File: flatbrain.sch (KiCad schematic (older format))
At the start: 89 parts, among them J1 OLED, J2 Conn_01x05, SW1 Rotary_Encoder_Switch, SW2 Rotary_Encoder_Switch, U1 Elite-C

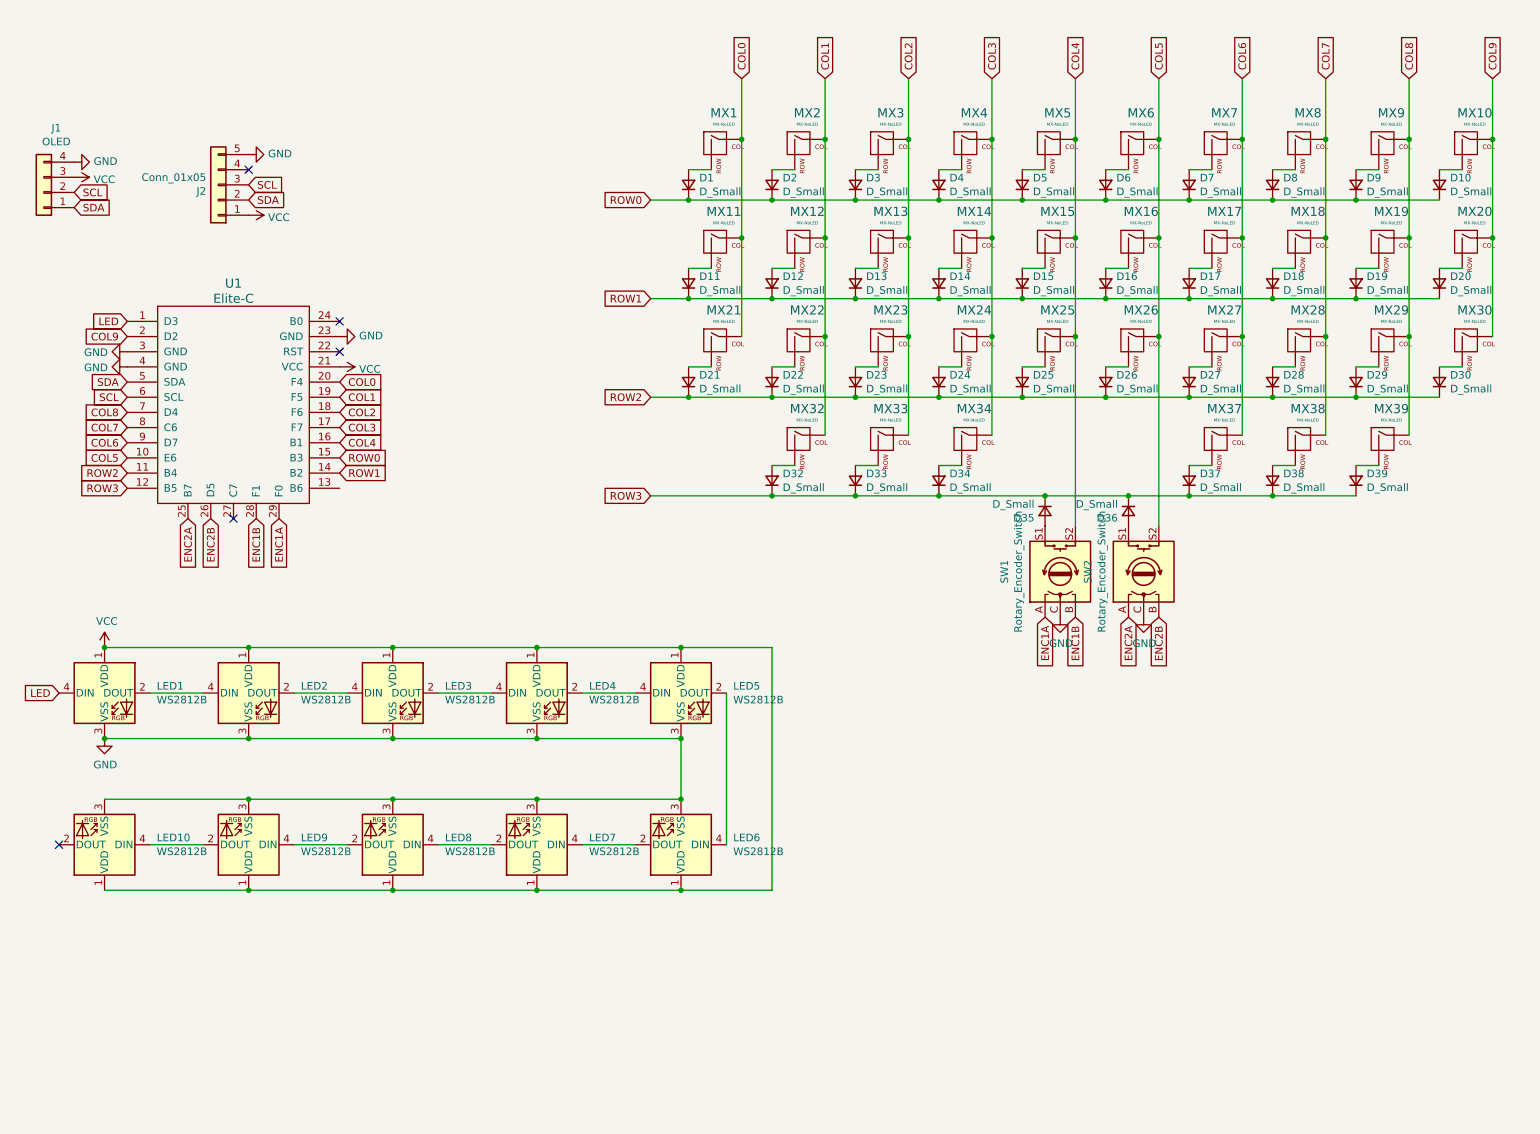
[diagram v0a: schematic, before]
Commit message: half pcba
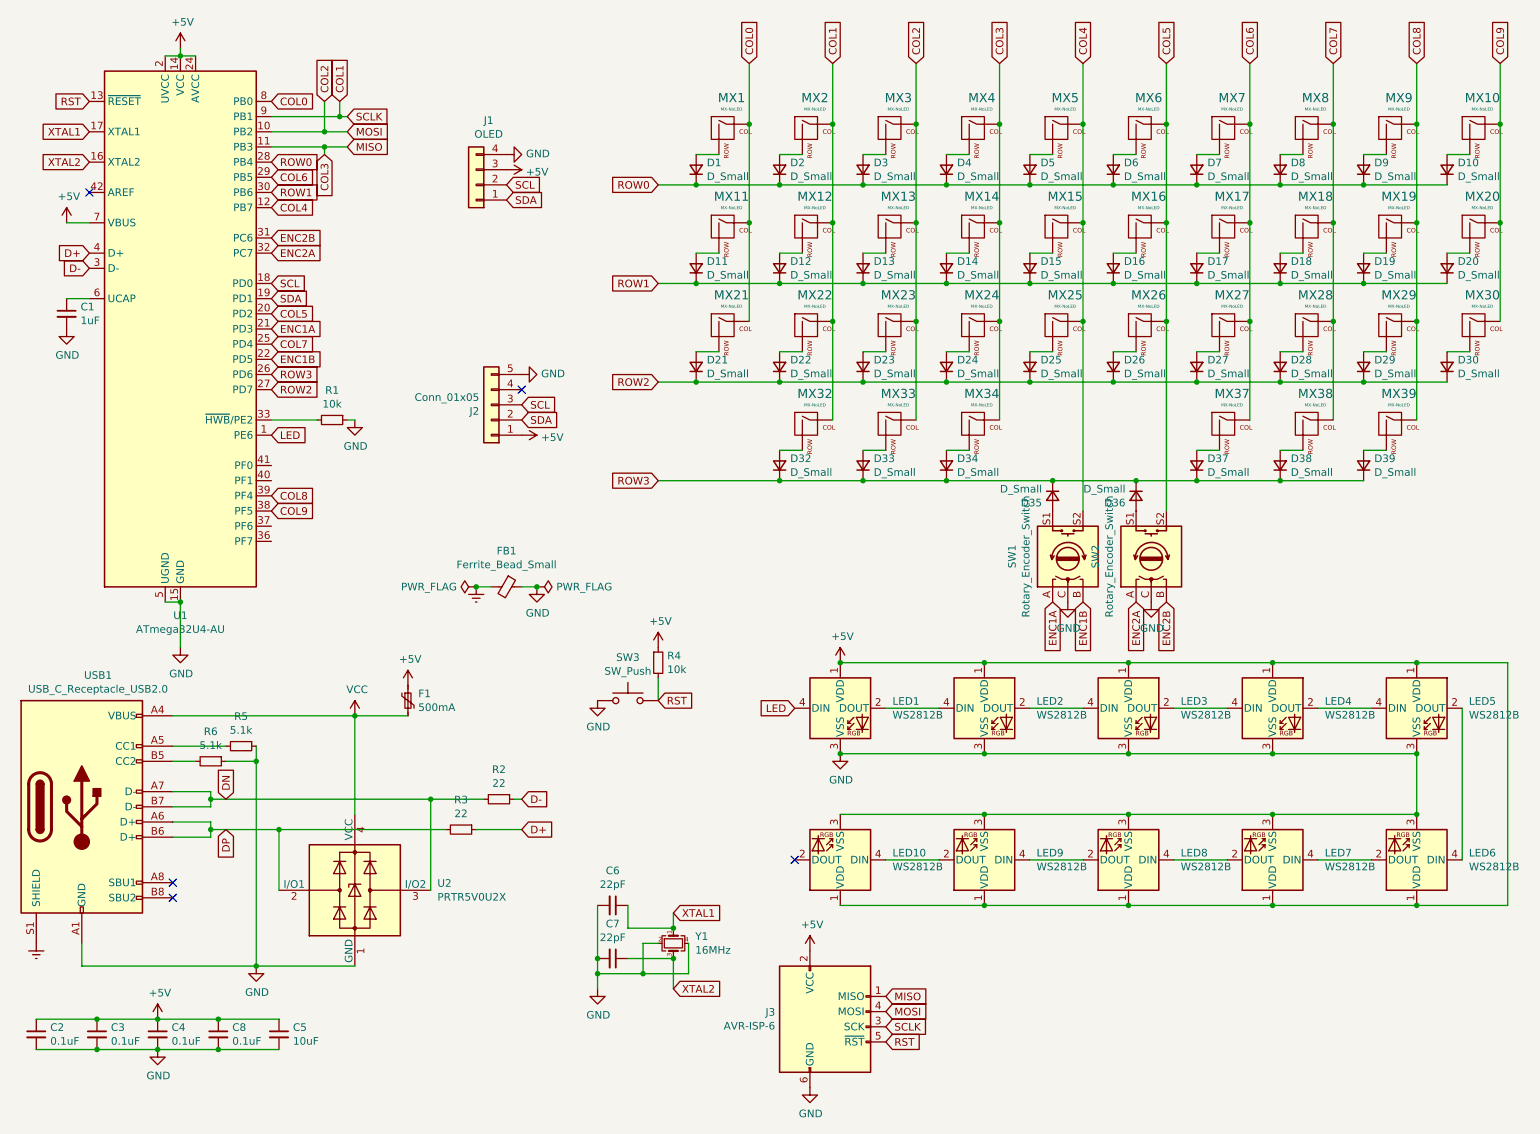
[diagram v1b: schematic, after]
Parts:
- removed U1: Elite-C, Keebio-Parts:Elite-C, symbol flatbrain:Elite-C
- added C1: 1uF, Capacitor_SMD:C_0805_2012Metric, symbol Device:C_Small
- added C2, C3, C4, C8: 0.1uF, Capacitor_SMD:C_0805_2012Metric, symbol Device:C_Small
- added C5: 10uF, Capacitor_SMD:C_0805_2012Metric, symbol Device:C_Small
- added C6, C7: 22pF, Capacitor_SMD:C_0805_2012Metric, symbol Device:C_Small
- added F1: 500mA, Fuse:Fuse_1206_3216Metric, symbol Device:Polyfuse_Small
- added FB1: Ferrite_Bead_Small, Inductor_SMD:L_0805_2012Metric_Pad1.15x1.40mm_HandSolder, symbol Device:Ferrite_Bead_Small
- added J3: AVR-ISP-6, random-keyboard-parts:Reset_Pretty-Mask, symbol Connector:AVR-ISP-6
- added R1, R4: 10k, Resistor_SMD:R_0805_2012Metric, symbol Device:R_Small
- added R2, R3: 22, Resistor_SMD:R_0805_2012Metric, symbol Device:R_Small
- added R5, R6: 5.1k, Resistor_SMD:R_0805_2012Metric, symbol Device:R_Small
- added SW3: SW_Push, random-keyboard-parts:SKQG-1155865, symbol Switch:SW_Push
- added U1: ATmega32U4-AU, Package_QFP:TQFP-44_10x10mm_P0.8mm, symbol MCU_Microchip_ATmega:ATmega32U4-AU
- added U2: PRTR5V0U2X, random-keyboard-parts:SOT143B, symbol Power_Protection:PRTR5V0U2X
- added USB1: USB_C_Receptacle_USB2.0, Connector_USB:USB_C_Receptacle_HRO_TYPE-C-31-M-12, symbol Connector:USB_C_Receptacle_USB2.0
- added Y1: 16MHz, Crystal:Crystal_SMD_3225-4Pin_3.2x2.5mm, symbol Device:Crystal_GND24_Small
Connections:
- net COL0: now also U1.8 (PB0)
- net COL1: now also J3.3 (SCK), U1.9 (PB1)
- net COL2: now also J3.4 (MOSI), U1.10 (PB2)
- net COL3: now also J3.1 (MISO), U1.11 (PB3)
- net COL4: now also U1.12 (PB7)
- net COL5: now also U1.20 (PD2)
- net COL6: now also U1.29 (PB5)
- net COL7: now also U1.25 (PD4)
- net COL8: now also U1.39 (PF4)
- net COL9: now also U1.38 (PF5)
- net ENC1A: now also U1.21 (PD3)
- net ENC1B: now also U1.22 (PD5)
- net ENC2A: now also U1.32 (PC7)
- net ENC2B: now also U1.31 (PC6)
- net GND: now also C1.2, C2.2, C3.2, C4.2, C5.2, C6.2, C7.2, C8.2, FB1.1, J3.6 (GND), R1.1, R5.1, R6.1, SW3.1, U1.15 (GND), U1.23 (GND), U1.35 (GND), U1.43 (GND), U1.5 (UGND), U2.1 (GND), USB1.A1 (GND), USB1.A12 (GND), USB1.B1 (GND), USB1.B12 (GND), Y1.2, Y1.4
- net LED: now also U1.1 (PE6)
- net ROW0: now also U1.28 (PB4)
- net ROW1: now also U1.30 (PB6)
- net ROW2: now also U1.27 (PD7)
- net ROW3: now also U1.26 (PD6)
- net SCL: now also U1.18 (PD0)
- net SDA: now also U1.19 (PD1)
- net VCC: now also F1.2, U2.4 (VCC), USB1.A4 (VBUS), USB1.A9 (VBUS), USB1.B4 (VBUS), USB1.B9 (VBUS); no longer J1.3 (Pin_3), J2.1 (Pin_1), LED1.1 (VDD), LED10.1 (VDD), LED2.1 (VDD), LED3.1 (VDD), LED4.1 (VDD), LED5.1 (VDD), LED6.1 (VDD), LED7.1 (VDD), LED8.1 (VDD), LED9.1 (VDD)
- new net: R1.2, U1.33 (~HWB~/PE2)
- new net: C1.1, U1.6 (UCAP)
- new net: R5.2, USB1.A5 (CC1)
- new net: R6.2, USB1.B5 (CC2)
- new net +5V: C2.1, C3.1, C4.1, C5.1, C8.1, F1.1, J1.3 (Pin_3), J2.1 (Pin_1), J3.2 (VCC), LED1.1 (VDD), LED10.1 (VDD), LED2.1 (VDD), LED3.1 (VDD), LED4.1 (VDD), LED5.1 (VDD), LED6.1 (VDD), LED7.1 (VDD), LED8.1 (VDD), LED9.1 (VDD), R4.1, U1.14 (VCC), U1.2 (UVCC), U1.24 (AVCC), U1.34 (VCC), U1.44 (AVCC), U1.7 (VBUS)
- new net D+: R3.1, U1.4 (D+)
- new net D-: R2.1, U1.3 (D-)
- new net DN: R2.2, U2.3 (I/O2), USB1.A7 (D-), USB1.B7 (D-)
- new net DP: R3.2, U2.2 (I/O1), USB1.A6 (D+), USB1.B6 (D+)
- new net Earth: FB1.2, USB1.S1 (SHIELD)
- new net RST: J3.5 (~RST), R4.2, SW3.2, U1.13 (~RESET)
- new net XTAL1: C6.1, U1.17 (XTAL1), Y1.1
- new net XTAL2: C7.1, U1.16 (XTAL2), Y1.3
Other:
- moved on the sheet: D1, D10, D11, D12, D13, D14, D15, D16, D17, D18, D19, D2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

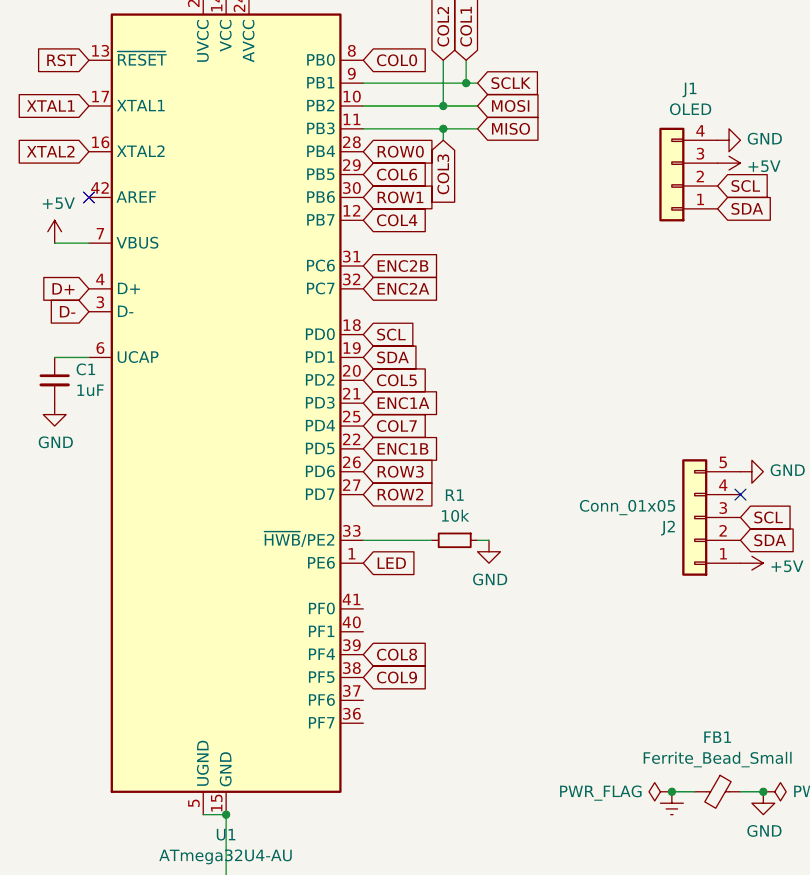
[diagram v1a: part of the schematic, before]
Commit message: pcba over
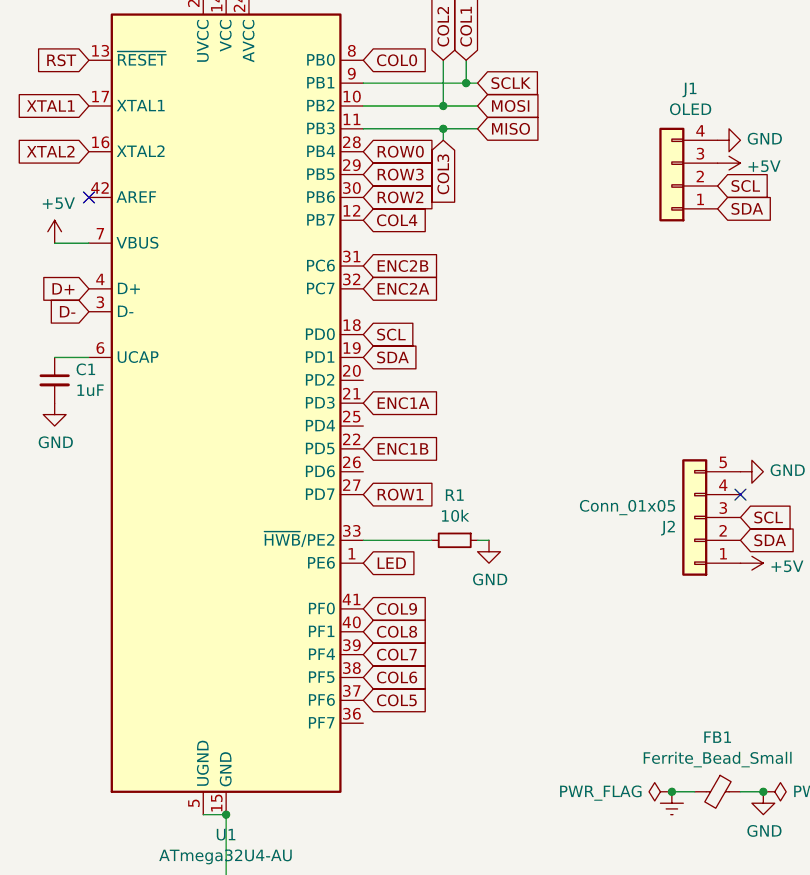
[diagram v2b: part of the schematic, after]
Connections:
- net COL5: now also U1.37 (PF6); no longer U1.20 (PD2)
- net COL6: now also U1.38 (PF5); no longer U1.29 (PB5)
- net COL7: now also U1.39 (PF4); no longer U1.25 (PD4)
- net COL8: now also U1.40 (PF1); no longer U1.39 (PF4)
- net COL9: now also U1.41 (PF0); no longer U1.38 (PF5)
- net ROW1: now also U1.27 (PD7); no longer U1.30 (PB6)
- net ROW2: now also U1.30 (PB6); no longer U1.27 (PD7)
- net ROW3: now also U1.29 (PB5); no longer U1.26 (PD6)
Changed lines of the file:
@@
 Text GLabel 2750 1400 3    50   Input ~ 0
 COL3
-Text GLabel 2400 2650 2    50   Input ~ 0
+Text GLabel 2400 3650 2    50   Input ~ 0
 COL7
-Text GLabel 2400 2950 2    50   Input ~ 0
+Text GLabel 2400 1650 2    50   Input ~ 0
 ROW2
 $Comp
@@
 Wire Wire Line
 	9400 3150 9400 2500
-Text GLabel 2400 2850 2    50   Input ~ 0
+Text GLabel 2400 1550 2    50   Input ~ 0
 ROW3
-Text GLabel 2400 1550 2    50   Input ~ 0
+Text GLabel 2400 3750 2    50   Input ~ 0
 COL6
 $Comp
@@
 Text GLabel 2400 1750 2    50   Input ~ 0
 COL4
-Text GLabel 2400 2450 2    50   Input ~ 0
+Text GLabel 2400 3850 2    50   Input ~ 0
 COL5
-Text GLabel 2400 3650 2    50   Input ~ 0
+Text GLabel 2400 3550 2    50   Input ~ 0
 COL8
-Text GLabel 2400 3750 2    50   Input ~ 0
+Text GLabel 2400 3450 2    50   Input ~ 0
 COL9
-Text GLabel 2400 1650 2    50   Input ~ 0
+Text GLabel 2400 2950 2    50   Input ~ 0
 ROW1
 Text GLabel 2400 2550 2    50   Input ~ 0
